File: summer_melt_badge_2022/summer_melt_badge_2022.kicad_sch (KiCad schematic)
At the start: 10 parts

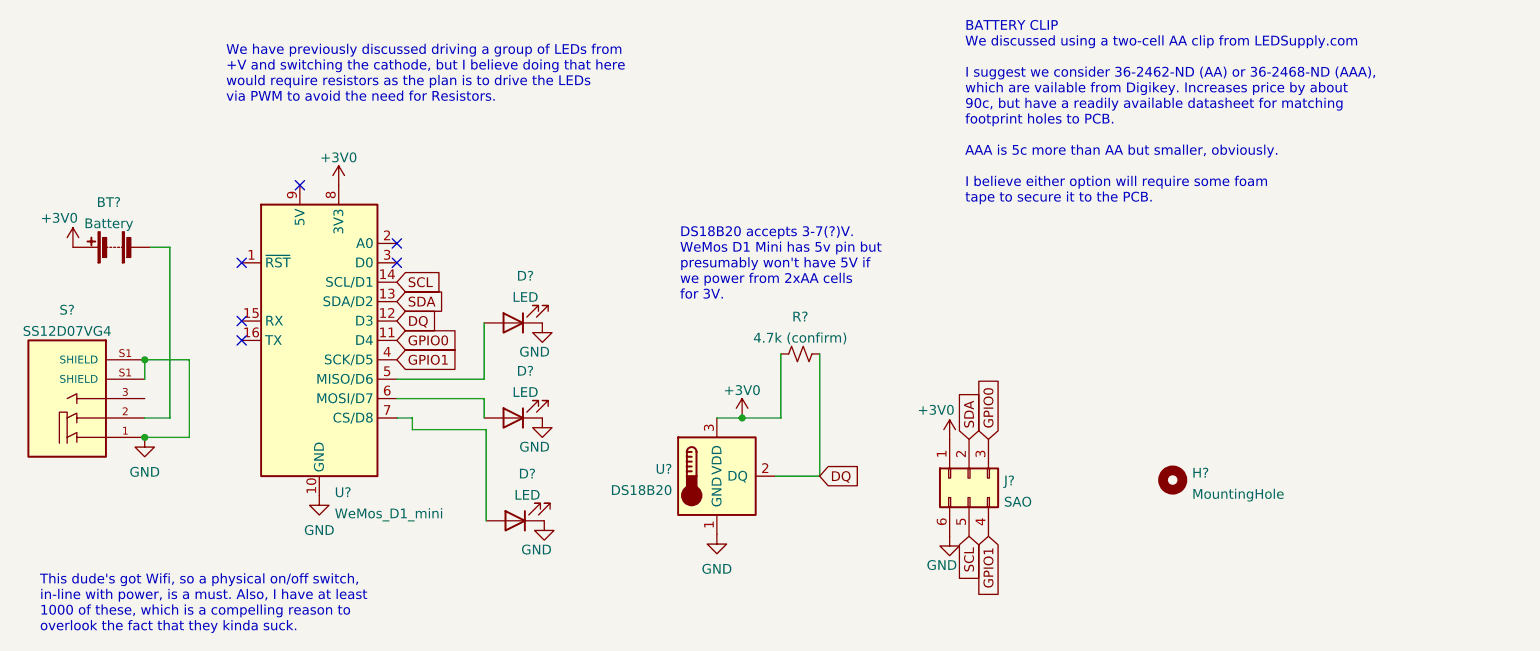
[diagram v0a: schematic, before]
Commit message: I made some changes to the schematic
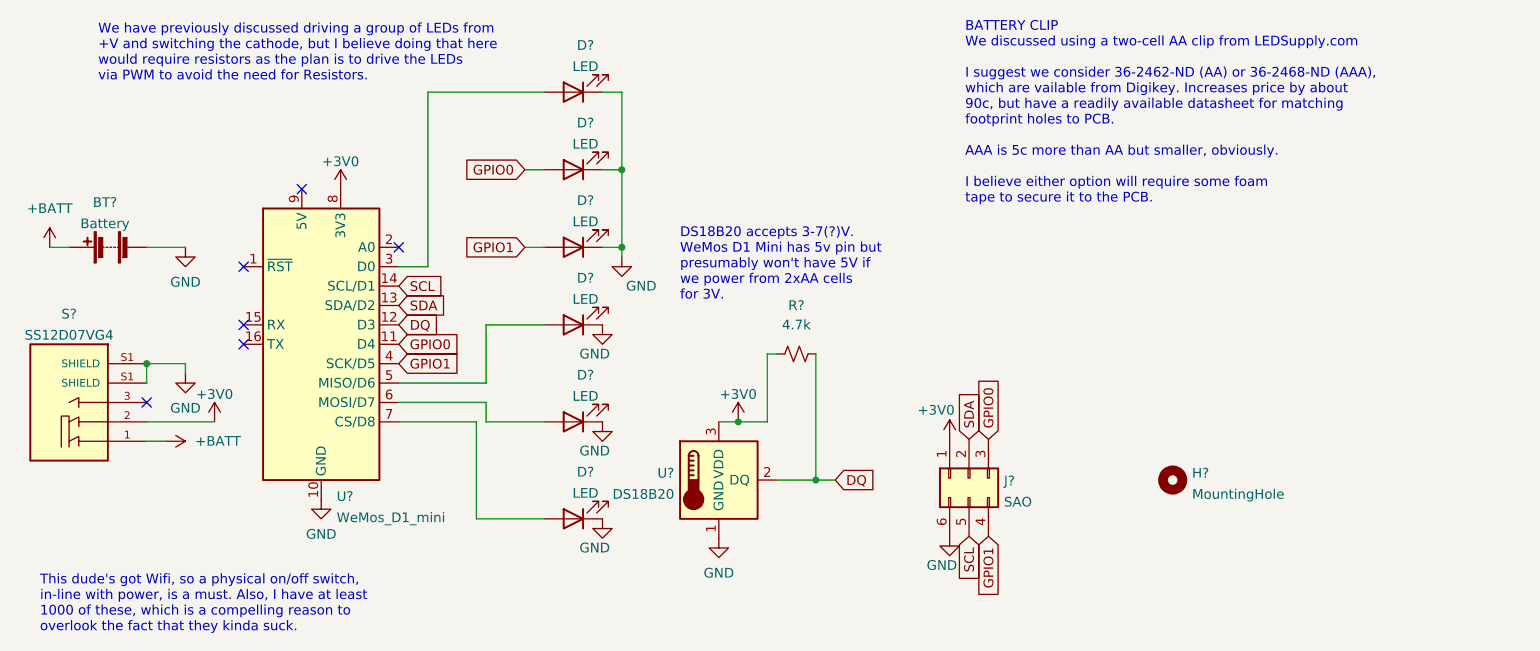
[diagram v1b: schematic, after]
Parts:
- added D? (x3): LED, symbol Device:LED
- R?: value 4.7k (confirm) -> 4.7k
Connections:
- net +3V0: now also S?.2; no longer BT?.1 (+)
- net GND: now also BT?.2 (-), D?.1 (K), D?.1 (K), D?.1 (K); no longer S?.1
- net GPIO0: now also D?.2 (A)
- net GPIO1: now also D?.2 (A)
- net at U?.3 (D0): now also D?.2 (A)
- new net +BATT: BT?.1 (+), S?.1
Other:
- moved on the sheet: BT?, D?, R?, S?, U?
